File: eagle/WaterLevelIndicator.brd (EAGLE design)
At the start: 52 x 75.9 mm, 7 parts, among them IC2 MAX7219CNG

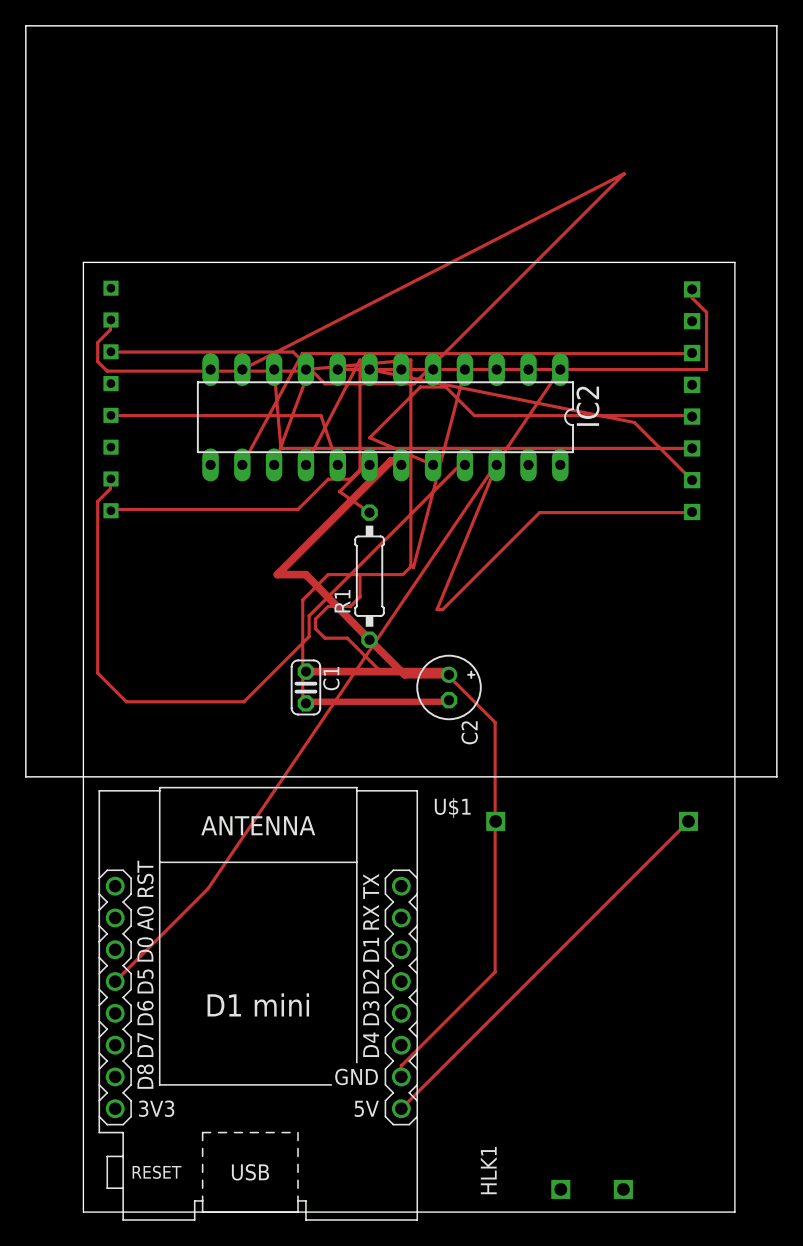
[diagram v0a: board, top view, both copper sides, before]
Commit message: more optimization
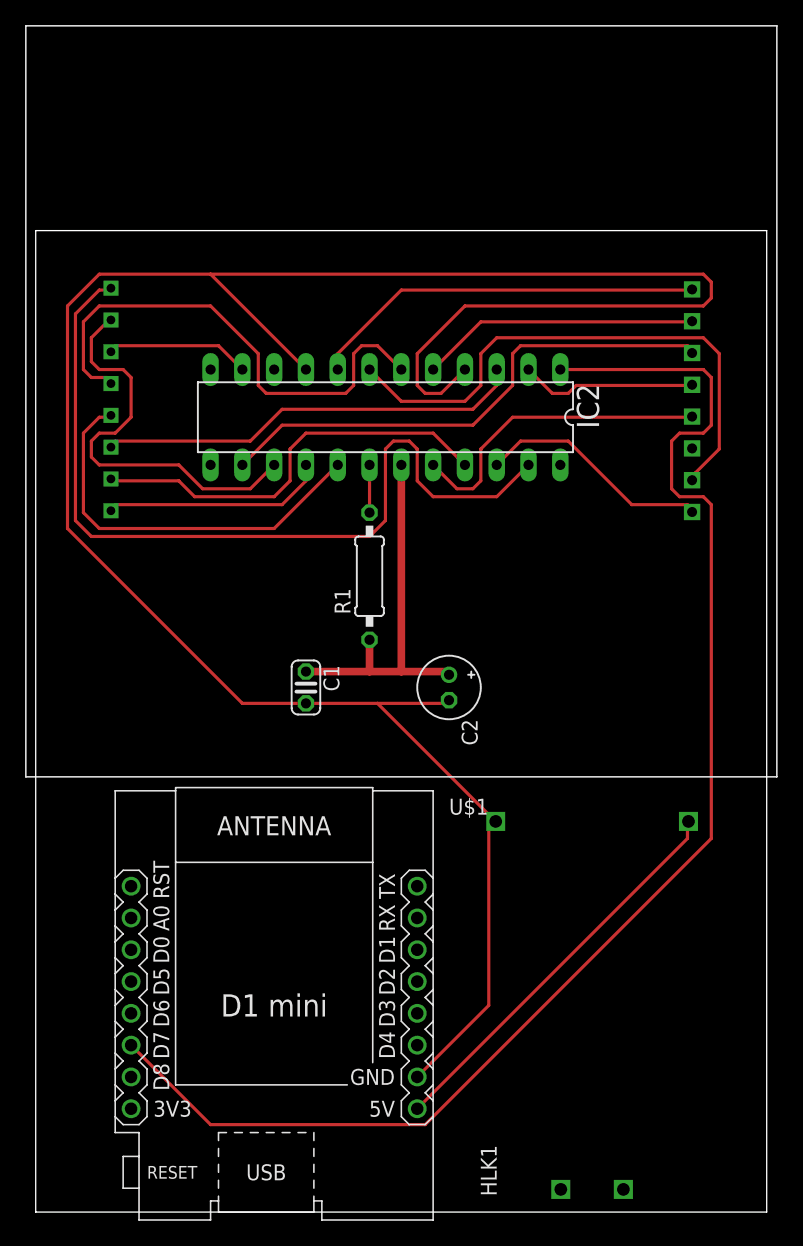
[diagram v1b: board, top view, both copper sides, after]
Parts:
- moved U$1 1.27 mm to (15.2, 40.6)
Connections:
- net N$4: now also U$1.JP1.6; no longer U$1.JP1.4
- net N$6: now also U$1.JP1.4; no longer U$1.JP1.6
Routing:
- net N$13: track 83.3 -> 11.5 mm
- net N$23: track 0.00 -> 67.8 mm
- net N$4: track 60.6 -> 112.5 mm
- net N$1: track 138.2 -> 188.4 mm
- net N$14: track 0.00 -> 40.7 mm
- net N$17: track 39.2 -> 0.00 mm
- net N$16: track 0.00 -> 34.2 mm
- net N$18: track 0.00 -> 22.3 mm
- net N$21: track 39.5 -> 17.9 mm
- net N$24: track 55.0 -> 33.5 mm
- net N$27: track 36.1 -> 18.8 mm
- net N$15: track 28.1 -> 44.1 mm
- net N$12: track 0.00 -> 14.1 mm
- net N$28: track 42.3 -> 30.7 mm
- net N$26: track 20.9 -> 32.1 mm
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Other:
- board size 52 x 75.9 mm -> 58.4 x 78.4 mm
